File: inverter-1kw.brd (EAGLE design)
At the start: 97.8 x 100.1 mm, 189 parts, among them IC1 LMV358MMX, IC2 LMV358MMX, Q4 1200980569**TRANS SMD NPN MMB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, Q6 1200980569**TRANS SMD NPN MMB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, U1 ACS712, U4 ACS712, U5 SI8230, U6 SI8230, U7 ACS712

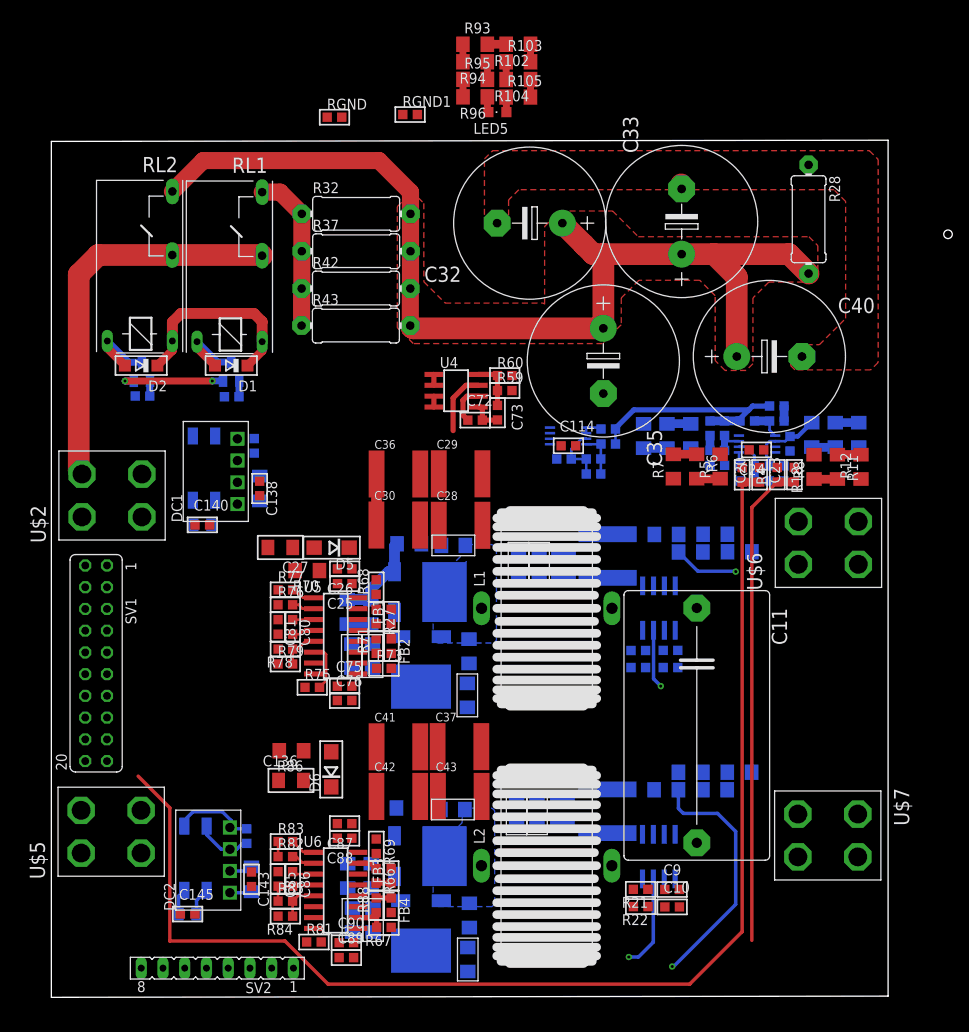
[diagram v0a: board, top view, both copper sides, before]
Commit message: Düzenlemeler yapıldı.
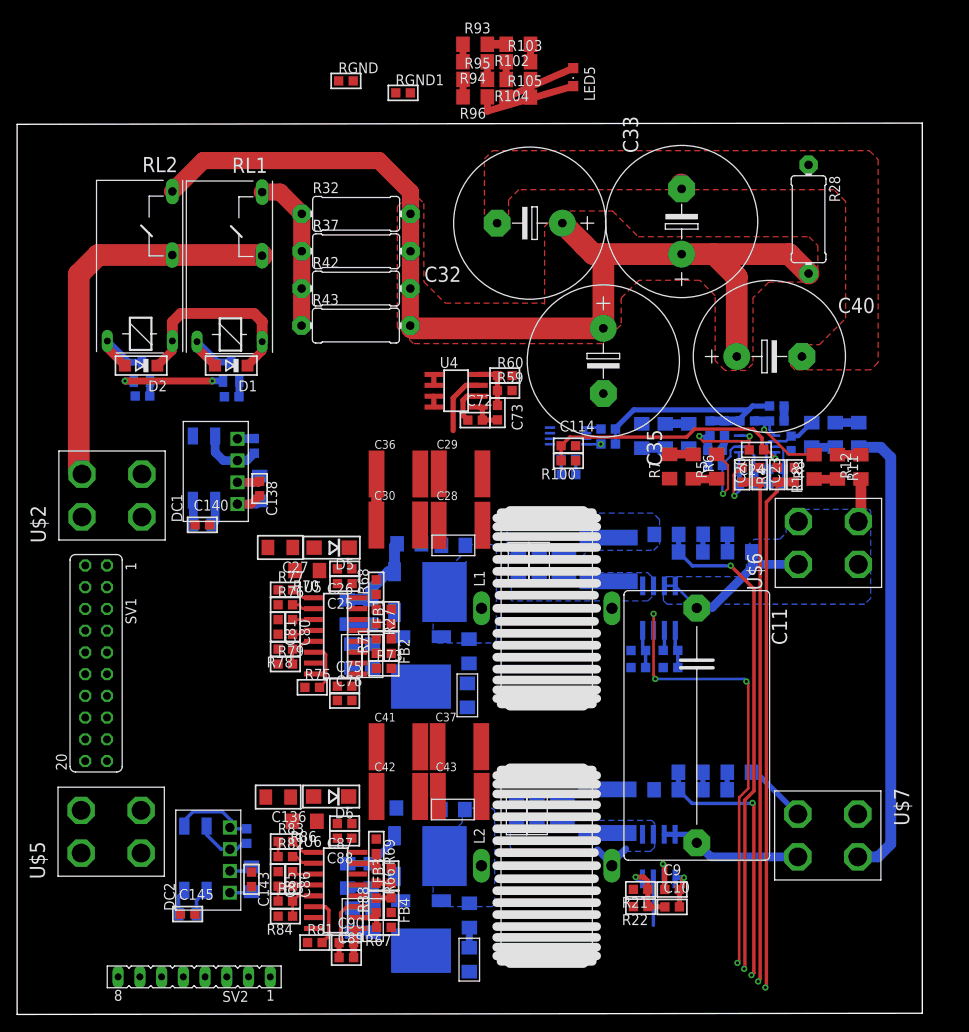
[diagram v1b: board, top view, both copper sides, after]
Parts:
- moved LED5 9.76 mm to (61.0, 107.5), turned to 180 degrees
- moved R86 8.38 mm to (29.6, 20.6)
- moved RGND 4.45 mm to (34.4, 107.1)
- moved D6 3.17 mm to (32.7, 23.5), turned to 180 degrees
- moved R101 2.95 mm to (60.4, 62.8)
- moved C19 2.93 mm to (60.4, 61.1)
- moved SV2 2.89 mm to (16.7, 2.39)
- moved RGND1 2.66 mm to (41.1, 105.7)
- moved C136 2.45 mm to (26.5, 23.4), turned to 180 degrees
- moved R100 0.55 mm to (60.4, 62.7), flipped to the top, turned to 180 degrees
- moved C4 0.45 mm to (59.9, 50.8)
- moved R7 0.43 mm to (72.2, 62.0)
- moved C1 0.42 mm to (65.1, 51.2)
- moved R6 0.41 mm to (75.0, 62.0)
- moved R5 0.40 mm to (77.7, 62.0)
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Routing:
- net VB_OUT: track 0.00 -> 78.0 mm
- net VOUT_SENS_DIFF: track 56.8 -> 109.4 mm, vias 0 -> 1
- net IB_SENS: track 85.4 -> 46.3 mm, vias 1 -> 0
- net VA_SENS: track 142.1 -> 103.6 mm, vias 1 -> 2
- net VIN_SENS_DIFF: track 146.9 -> 110.3 mm, vias 0 -> 1
- net +3V3: track 0.00 -> 30.8 mm, vias 0 -> 1
- net VA_OUT: track 0.00 -> 26.6 mm
- net DGND: track 37.8 -> 62.0 mm, vias 2 -> 6
- net AGND: track 2.38 -> 18.7 mm
- net N$9: track 5.19 -> 17.6 mm, vias 0 -> 1
- net IA_SENS: track 128.6 -> 139.7 mm, vias 1 -> 4
- net N$20: track 3.73 -> 12.0 mm, vias 0 -> 1
- net VCC_2: track 3.05 -> 10.7 mm
- net N$95: track 0.00 -> 7.55 mm
- net N$18: track 1.65 -> 9.18 mm, vias 0 -> 1
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- added copper zone on layer 16, net AGND
- added copper zone on layer 16, net VA_FILTER
- added copper zone on layer 16, net VA_OUT
- added copper zone on layer 16, net VB_FILTER
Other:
- board size 97.8 x 100.1 mm -> 105.8 x 104.1 mm
